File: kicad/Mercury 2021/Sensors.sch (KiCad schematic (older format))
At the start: 10 parts

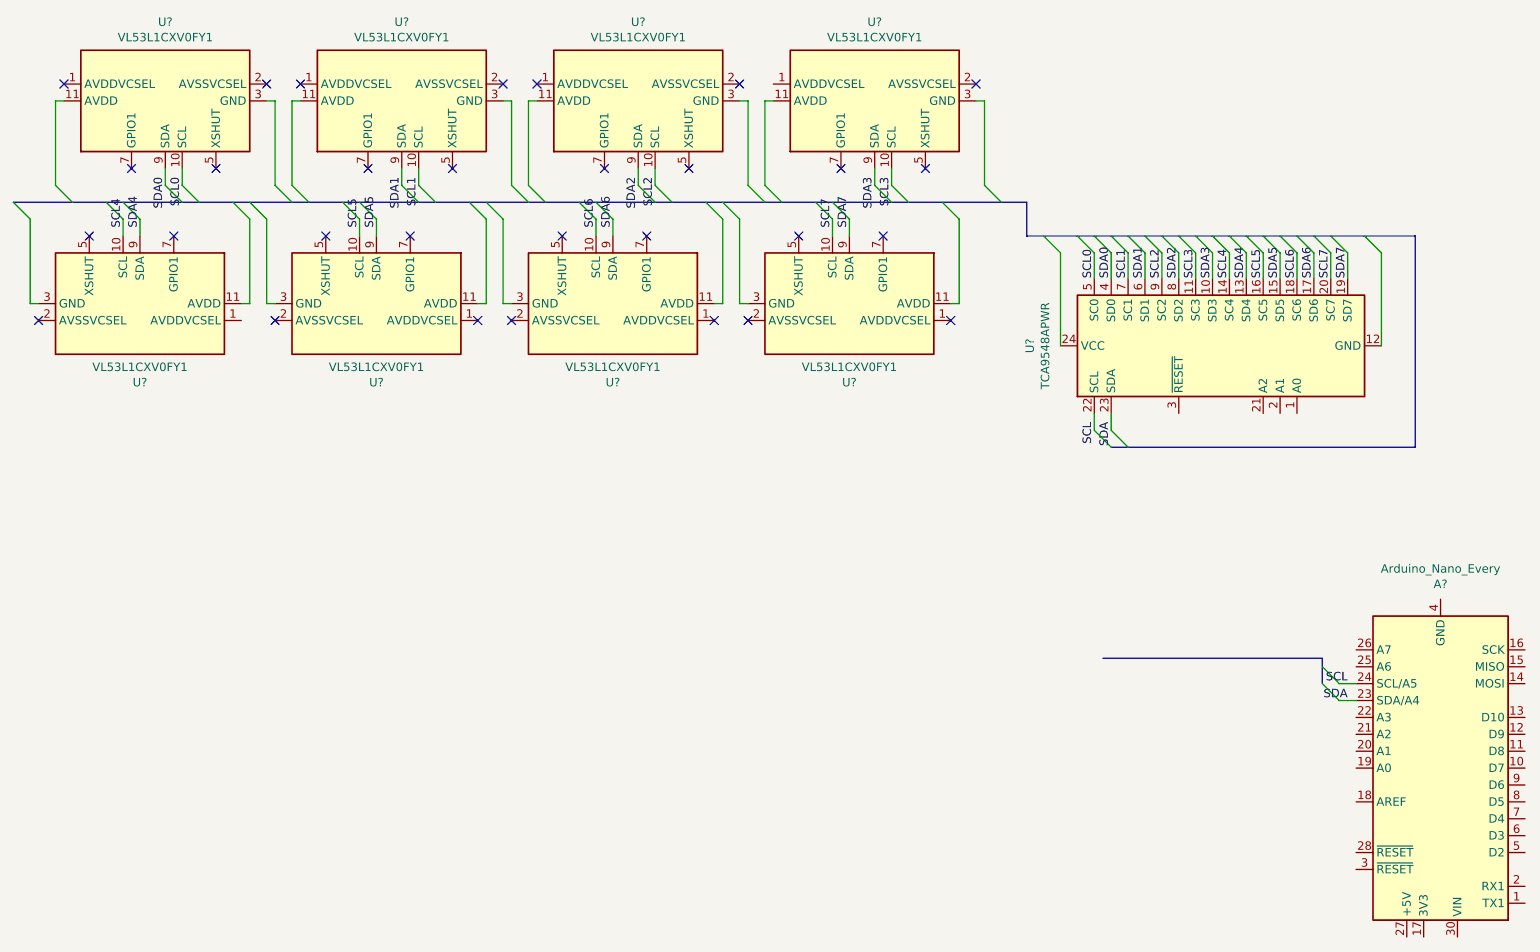
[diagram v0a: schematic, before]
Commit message: Updated new board
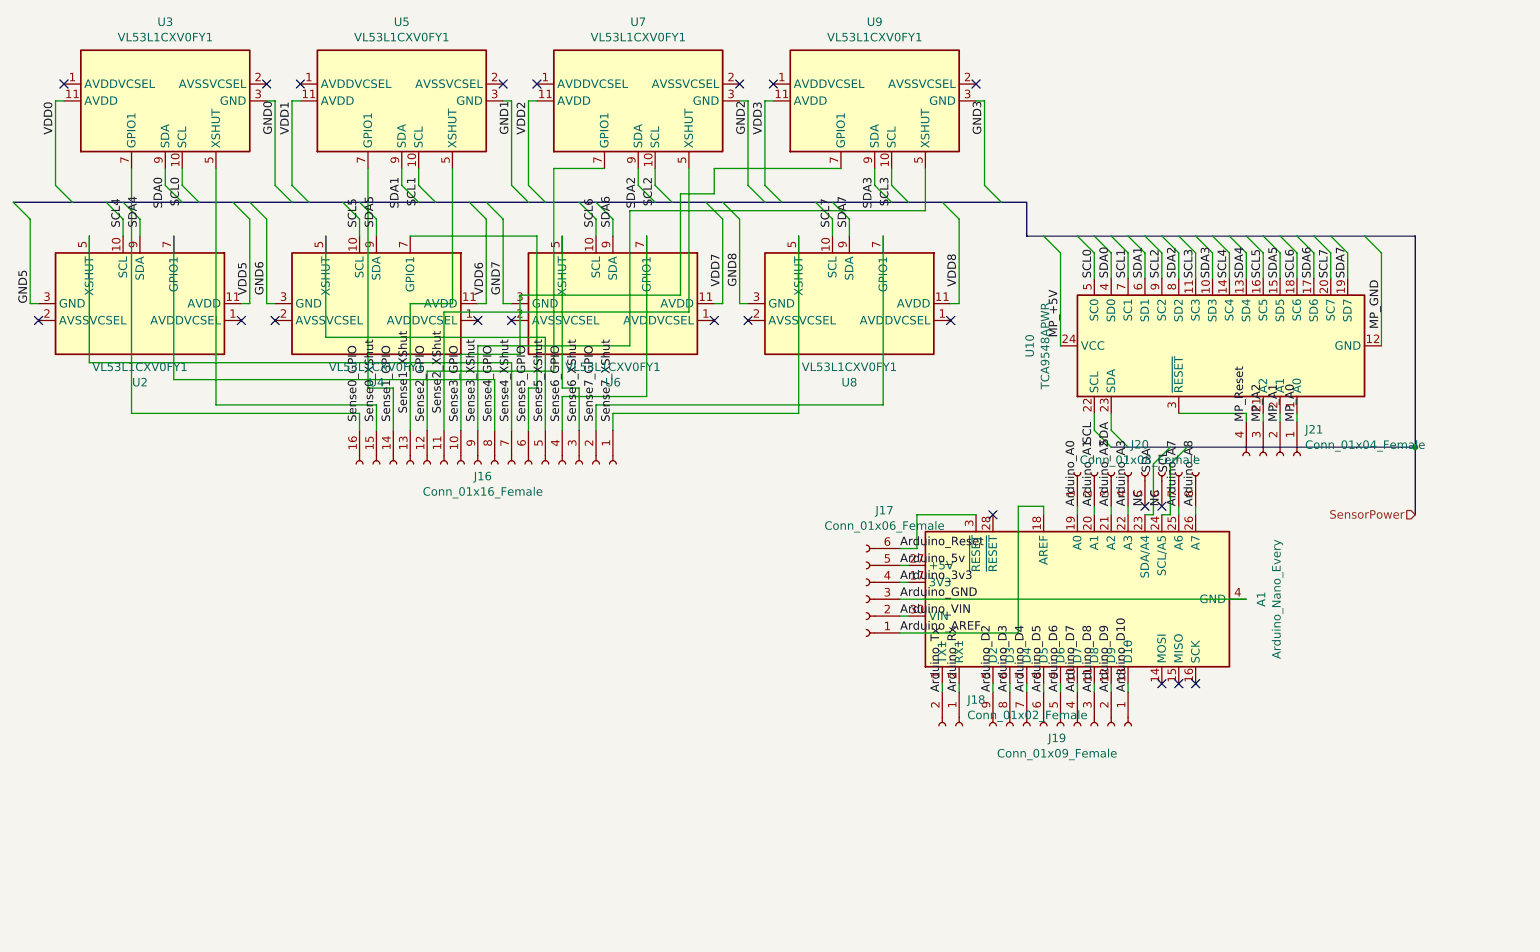
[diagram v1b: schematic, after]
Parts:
- added J16: Conn_01x16_Female, symbol Connector:Conn_01x16_Female
- added J17: Conn_01x06_Female, symbol Connector:Conn_01x06_Female
- added J18: Conn_01x02_Female, symbol Connector:Conn_01x02_Female
- added J19: Conn_01x09_Female, symbol Connector:Conn_01x09_Female
- added J20: Conn_01x08_Female, symbol Connector:Conn_01x08_Female
- added J21: Conn_01x04_Female, symbol Connector:Conn_01x04_Female
- U2, U3, U4, U5, U6, U7, U8, U9: renamed from U?; footprint Sensor_Distance:ST_VL53L1x -> Connector_PinHeader_2.54mm:PinHeader_1x06_P2.54mm_Vertical
- gave numbers to parts that had none: 2
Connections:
- net MP_A0: now reaches U10.1 (A0)
- net MP_A0: now also J21.1 (Pin_1)
- net MP_GND: now reaches U10.12 (GND)
- net MP_A1: now reaches U10.2 (A1)
- net MP_A1: now also J21.2 (Pin_2)
- net MP_A2: now reaches U10.21 (A2)
- net MP_A2: now also J21.3 (Pin_3)
- net MP_+5V: now reaches U10.24 (VCC)
- net MP_Reset: now reaches U10.3 (~RESET)
- net MP_Reset: now also J21.4 (Pin_4)
- net Arduino_Tx: now reaches A1.1 (TX1)
- net Arduino_Tx: now also J18.2 (Pin_2)
- net Arduino_D7: now reaches A1.10 (D7)
- net Arduino_D7: now also J19.4 (Pin_4)
- net Arduino_D8: now reaches A1.11 (D8)
- net Arduino_D8: now also J19.3 (Pin_3)
- net Arduino_D9: now reaches A1.12 (D9)
- net Arduino_D9: now also J19.2 (Pin_2)
- net Arduino_D10: now reaches A1.13 (D10)
- net Arduino_D10: now also J19.1 (Pin_1)
- net Arduino_3v3: now reaches A1.17 (3V3)
- net Arduino_3v3: now also J17.4 (Pin_4)
- net Arduino_AREF: now reaches A1.18 (AREF)
- net Arduino_AREF: now also J17.1 (Pin_1)
- net Arduino_A0: now reaches A1.19 (A0)
- net Arduino_A0: now also J20.1 (Pin_1)
- net Arduino_Rx: now reaches A1.2 (RX1)
- net Arduino_Rx: now also J18.1 (Pin_1)
- net Arduino_A1: now reaches A1.20 (A1)
- net Arduino_A1: now also J20.2 (Pin_2)
- net Arduino_A2: now reaches A1.21 (A2)
- net Arduino_A2: now also J20.3 (Pin_3)
- net Arduino_A3: now reaches A1.22 (A3)
- net Arduino_A3: now also J20.4 (Pin_4)
- net Arduino_A7: now reaches A1.25 (A6)
- net Arduino_A7: now also J20.7 (Pin_7)
- net Arduino_A8: now reaches A1.26 (A7)
- net Arduino_A8: now also J20.8 (Pin_8)
- net Arduino_5v: now reaches A1.27 (+5V)
- net Arduino_5v: now also J17.5 (Pin_5)
- net Arduino_GND: now reaches A1.29 (GND), A1.4 (GND)
- net Arduino_GND: now also J17.3 (Pin_3)
- net Arduino_Reset: now reaches A1.3 (~RESET)
- net Arduino_Reset: now also J17.6 (Pin_6)
- net Arduino_VIN: now reaches A1.30 (VIN)
- net Arduino_VIN: now also J17.2 (Pin_2)
- net Arduino_D2: now reaches A1.5 (D2)
- net Arduino_D2: now also J19.9 (Pin_9)
- net Arduino_D3: now reaches A1.6 (D3)
- net Arduino_D3: now also J19.8 (Pin_8)
- net Arduino_D4: now reaches A1.7 (D4)
- net Arduino_D4: now also J19.7 (Pin_7)
- net Arduino_D5: now reaches A1.8 (D5)
- net Arduino_D5: now also J19.6 (Pin_6)
- net Arduino_D6: now reaches A1.9 (D6)
- net Arduino_D6: now also J19.5 (Pin_5)
- net VDD0: now reaches U3.11 (AVDD)
- net GND0: now reaches U3.12 (GND), U3.3 (GND), U3.4 (GND), U3.6 (GND)
- net Sense0_XShut: now reaches U3.5 (XSHUT)
- net Sense0_XShut: now also J16.15 (Pin_15)
- net Sense0_GPIO: now reaches U3.7 (GPIO1)
- net Sense0_GPIO: now also J16.16 (Pin_16)
- net VDD1: now reaches U5.11 (AVDD)
- net GND1: now reaches U5.12 (GND), U5.3 (GND), U5.4 (GND), U5.6 (GND)
- net Sense1_XShut: now reaches U5.5 (XSHUT)
- net Sense1_XShut: now also J16.13 (Pin_13)
- net Sense1_GPIO: now reaches U5.7 (GPIO1)
- net Sense1_GPIO: now also J16.14 (Pin_14)
- net VDD2: now reaches U7.11 (AVDD)
- net GND2: now reaches U7.12 (GND), U7.3 (GND), U7.4 (GND), U7.6 (GND)
- net Sense2_XShut: now reaches U7.5 (XSHUT)
- net Sense2_XShut: now also J16.11 (Pin_11)
- net Sense2_GPIO: now reaches U7.7 (GPIO1)
- net Sense2_GPIO: now also J16.12 (Pin_12)
- net VDD3: now reaches U9.11 (AVDD)
- net GND3: now reaches U9.12 (GND), U9.3 (GND), U9.4 (GND), U9.6 (GND)
- net Sense3_XShut: now reaches U9.5 (XSHUT)
- net Sense3_XShut: now also J16.9 (Pin_9)
- net Sense3_GPIO: now reaches U9.7 (GPIO1)
- net Sense3_GPIO: now also J16.10 (Pin_10)
- net VDD8: now reaches U8.11 (AVDD)
- net GND8: now reaches U8.12 (GND), U8.3 (GND), U8.4 (GND), U8.6 (GND)
- net Sense7_XShut: now reaches U8.5 (XSHUT)
- net Sense7_XShut: now also J16.1 (Pin_1)
- net Sense7_GPIO: now reaches U8.7 (GPIO1)
- net Sense7_GPIO: now also J16.2 (Pin_2)
- net VDD7: now reaches U6.11 (AVDD)
- net GND7: now reaches U6.12 (GND), U6.3 (GND), U6.4 (GND), U6.6 (GND)
- net Sense6_XShut: now reaches U6.5 (XSHUT)
- net Sense6_XShut: now also J16.3 (Pin_3)
- net Sense6_GPIO: now reaches U6.7 (GPIO1)
- net Sense6_GPIO: now also J16.4 (Pin_4)
- net VDD6: now reaches U4.11 (AVDD)
- net GND6: now reaches U4.12 (GND), U4.3 (GND), U4.4 (GND), U4.6 (GND)
- net Sense5_XShut: now reaches U4.5 (XSHUT)
- net Sense5_XShut: now also J16.5 (Pin_5)
- net Sense5_GPIO: now reaches U4.7 (GPIO1)
- net Sense5_GPIO: now also J16.6 (Pin_6)
- net VDD5: now reaches U2.11 (AVDD)
- net GND5: now reaches U2.12 (GND), U2.3 (GND), U2.4 (GND), U2.6 (GND)
- net Sense4_XShut: now reaches U2.5 (XSHUT)
- net Sense4_XShut: now also J16.7 (Pin_7)
- net Sense4_GPIO: now reaches U2.7 (GPIO1)
- net Sense4_GPIO: now also J16.8 (Pin_8)
- new net NC: J20.5 (Pin_5), J20.6 (Pin_6)
- no-connect marks 30 -> 22
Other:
- moved on the sheet: A1
